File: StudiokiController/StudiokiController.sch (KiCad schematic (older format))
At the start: 59 parts, among them J1 USB_B_Micro, J10 Conn_01x10_Male, J11 Screw_Terminal_01x03, J12 Screw_Terminal_01x02, J2 Screw_Terminal_01x03, J3 Conn_01x04_Female, J4 57PC5FS, J5 Conn_01x02_Female, J6 Screw_Terminal_01x03, J7 Screw_Terminal_01x03, J8 Conn_01x03_Female, Q1 Q_DUAL_NPN_NPN_E1B1C2E2B2C1, SW1 SW_Push, SW2 SW_Push, SW3 SW_Push, U1 CH340C, U2 ESP32-WROOM-32D, U3 MAX31855KASA, U4 AZ1117-3.3, U5 MAX31865AAP+T

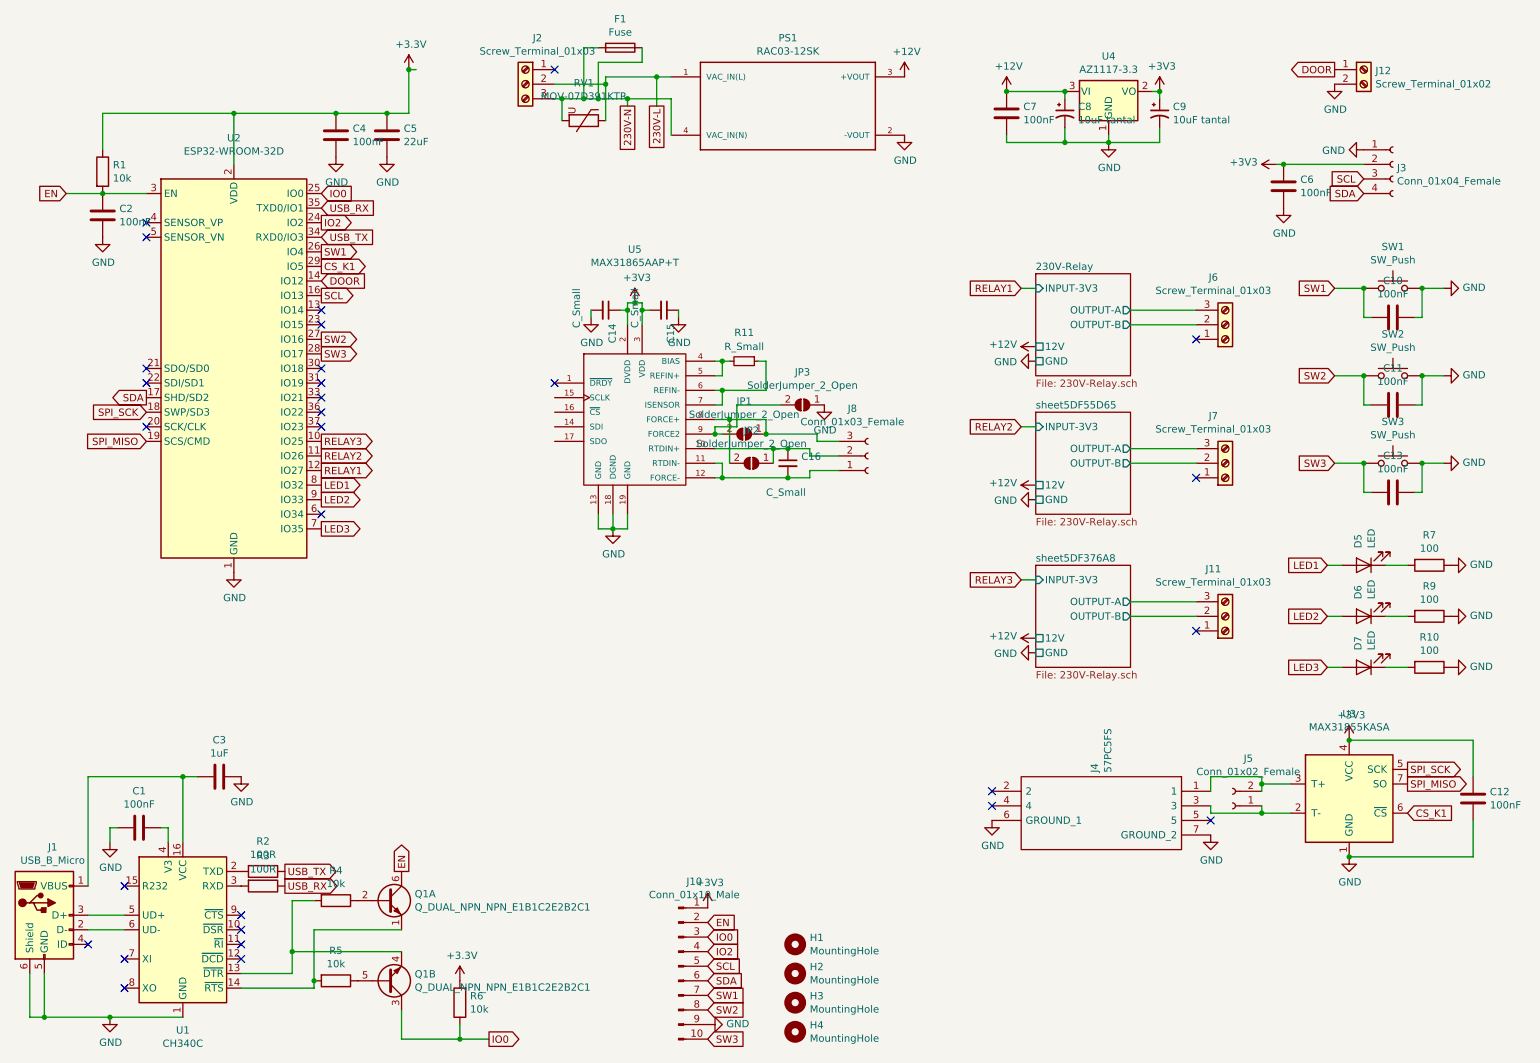
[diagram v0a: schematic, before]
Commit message: gjkl
fh
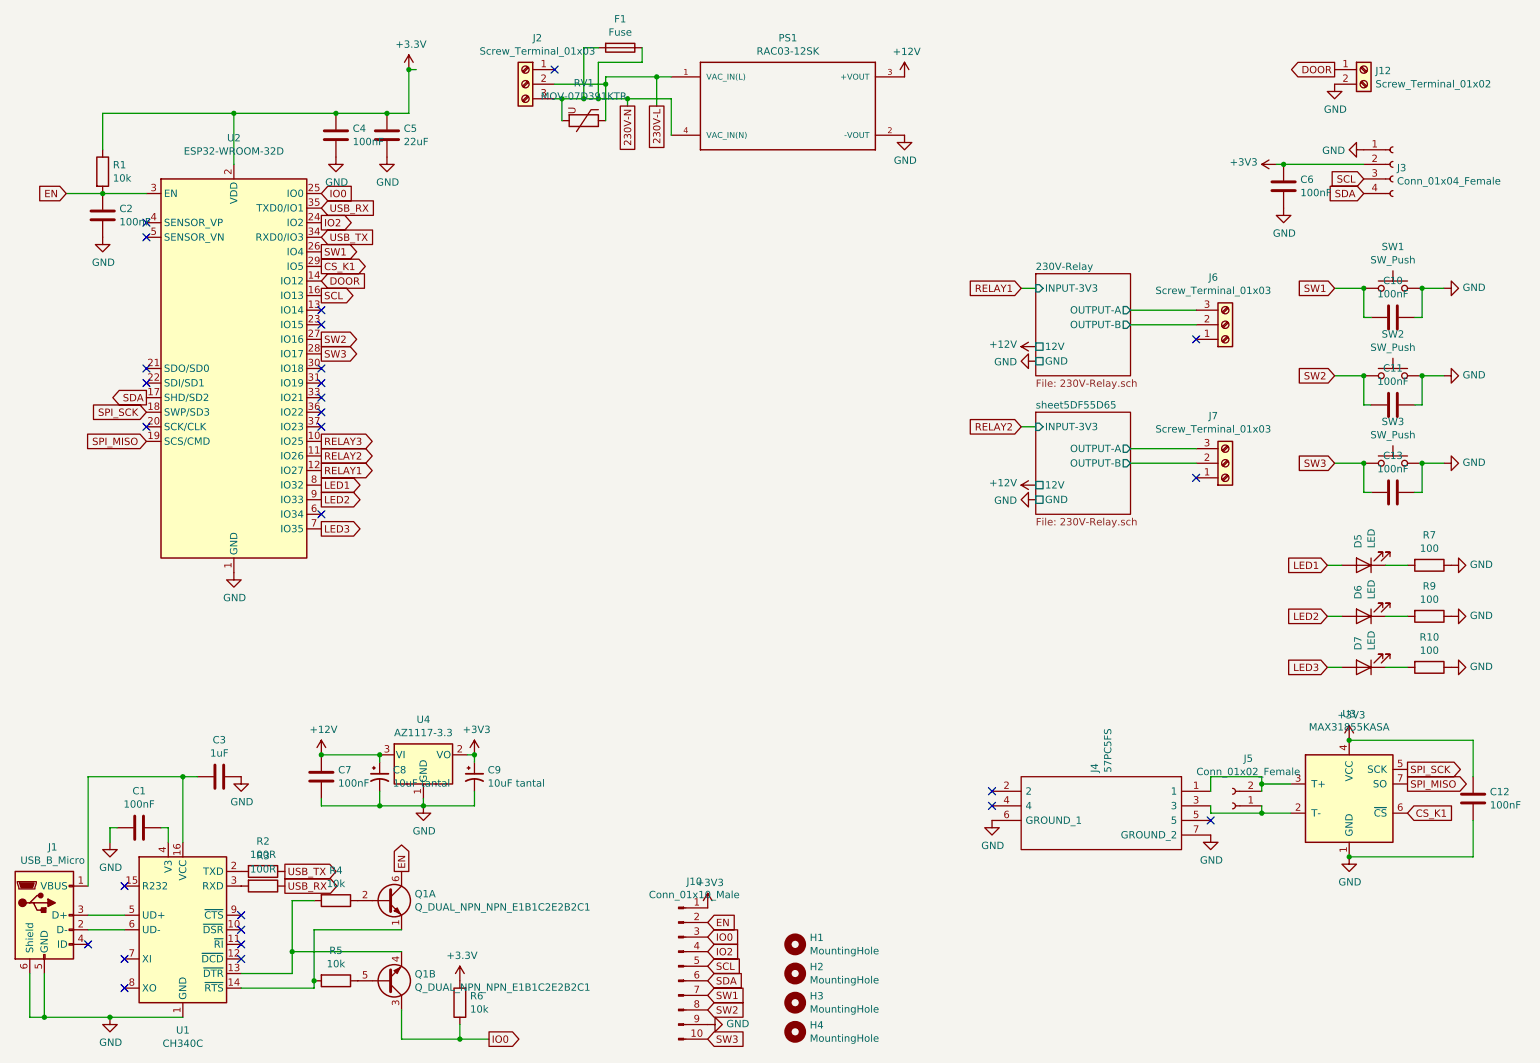
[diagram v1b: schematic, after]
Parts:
- removed C14, C15, C16: C_Small, Capacitor_SMD:C_0603_1608Metric, symbol Device:C_Small
- removed J11: Screw_Terminal_01x03, TerminalBlock_Phoenix:TerminalBlock_Phoenix_PT-1,5-3-5.0-H_1x03_P5.00mm_Horizontal, symbol Connector:Screw_Terminal_01x03
- removed J8: Conn_01x03_Female, StudiokiController:WAGO2060-473-998-404, symbol Connector:Conn_01x03_Female
- removed JP1, JP2, JP3: SolderJumper_2_Open, Jumper:SolderJumper-2_P1.3mm_Open_RoundedPad1.0x1.5mm, symbol Jumper:SolderJumper_2_Open
- removed R11: R_Small, Resistor_SMD:R_0603_1608Metric, symbol Device:R_Small
- removed U5: MAX31865AAP+T, SOP65P777X199-20N, symbol MAX31865AAP_T:MAX31865AAP+T
- J1: footprint (none) -> Connector_USB:USB_Micro-B_Molex-105017-0001
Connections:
- no-connect marks 29 -> 27
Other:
- moved on the sheet: C7, C8, C9, U4
